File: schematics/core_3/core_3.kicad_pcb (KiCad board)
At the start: 2 copper layers, 100 x 91.1 mm, 14 parts

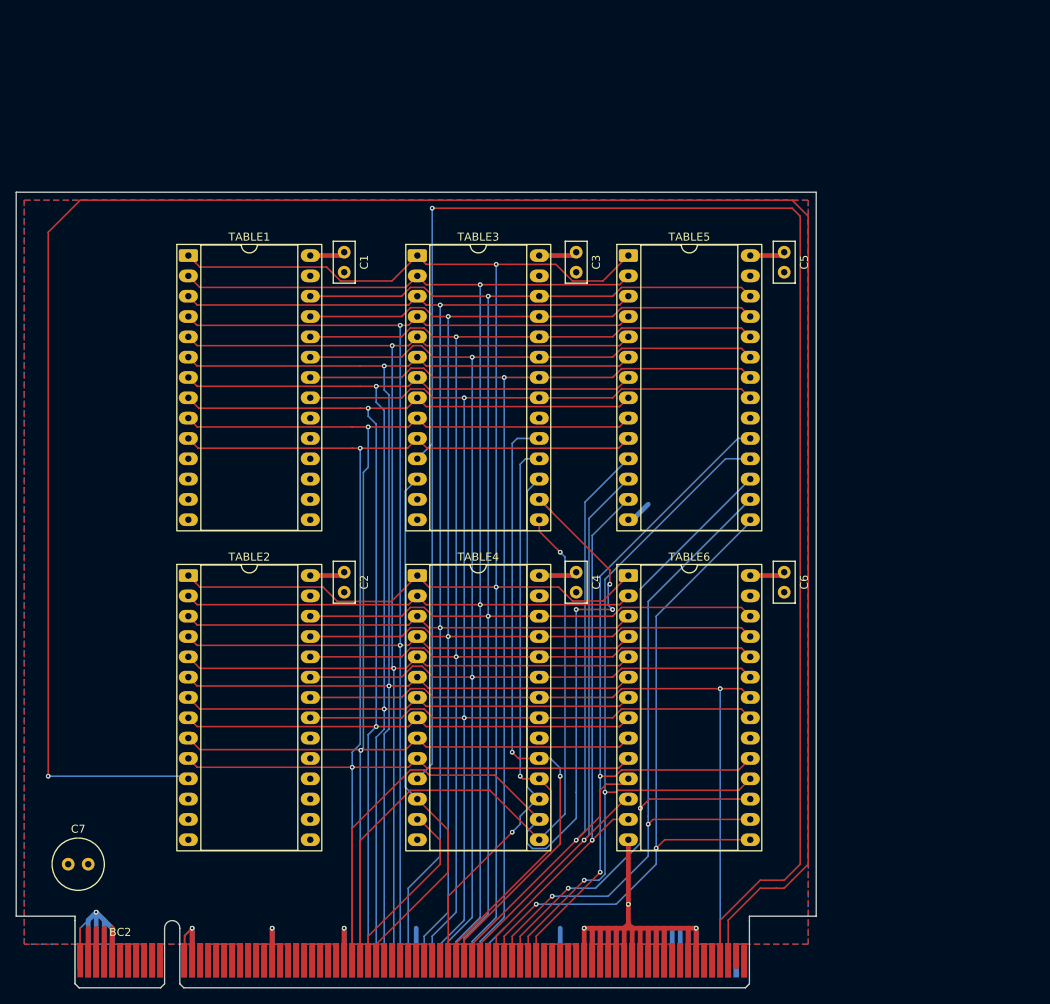
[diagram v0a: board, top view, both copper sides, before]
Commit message: tried to make core_3
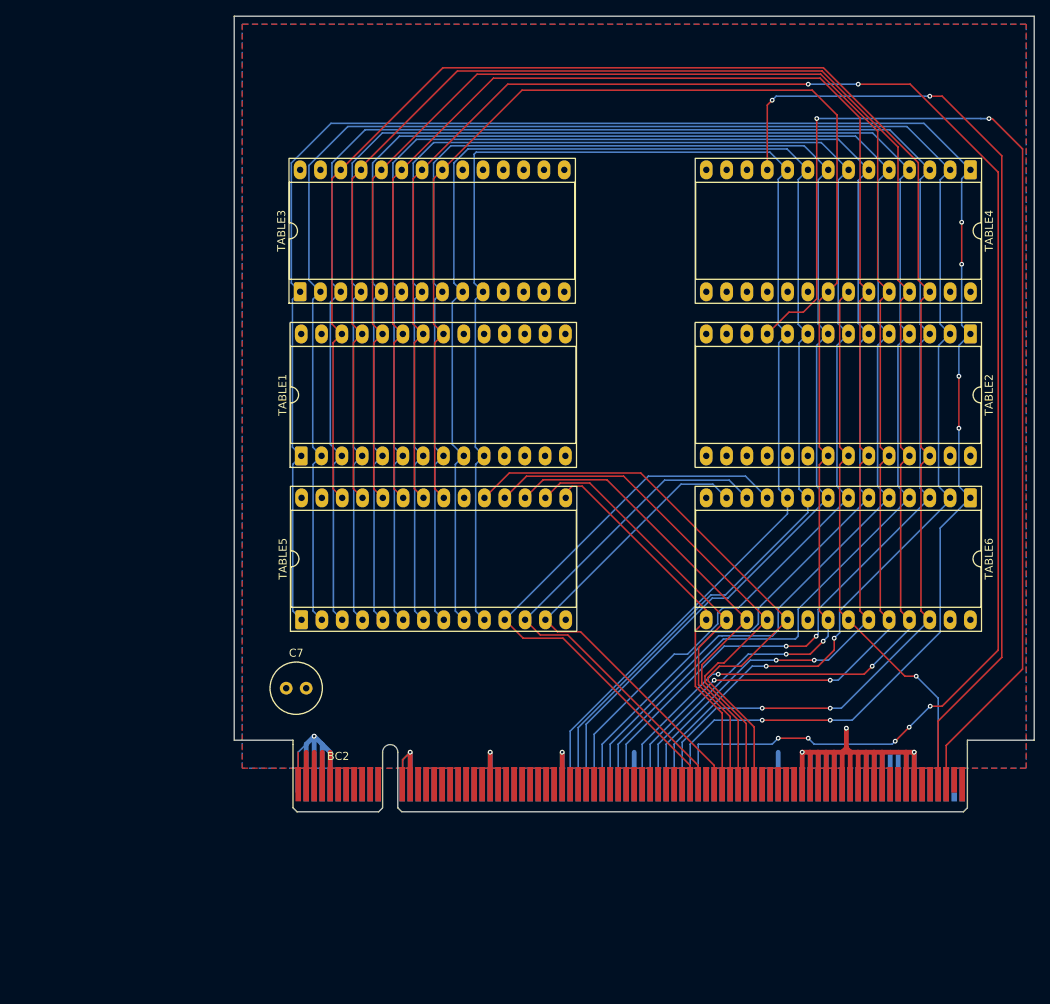
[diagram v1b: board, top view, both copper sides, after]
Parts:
- removed C1, C2, C3, C4, C5, C6: C, Capacitor_THT:C_Disc_D5.0mm_W2.5mm_P2.50mm
- moved TABLE2 102.3 mm to (172.3, 70.7), turned to -90 degrees
- moved TABLE4 85.7 mm to (172.3, 50.2), turned to -90 degrees
- moved TABLE5 61.2 mm to (88.7, 106.4), turned to 90 degrees
- moved TABLE6 43.8 mm to (172.3, 91.2), turned to -90 degrees
- moved BC2 35.0 mm to (88.2, 127.0)
- moved C7 35.0 mm to (86.8, 115.0)
- moved TABLE1 28.7 mm to (88.6, 86.0), turned to 90 degrees
- moved TABLE3 15.3 mm to (88.5, 65.4), turned to 90 degrees
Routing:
- net Net-(BC2-R4): track 282.0 -> 141.2 mm, vias 1 -> 2
- net Net-(BC2-L0): track 107.7 -> 0.00 mm, vias 3 -> 0
- net /STATE15: track 131.0 -> 233.6 mm, vias 1 -> 7
- net Net-(BC2-L4): track 220.0 -> 122.8 mm, vias 1 -> 2
- net Net-(BC2-L1): track 85.2 -> 0.00 mm, vias 1 -> 0
- net /PCIncrement: track 78.0 -> 0.00 mm, vias 2 -> 0
- net /~{Halt}: track 72.4 -> 0.00 mm, vias 1 -> 0
- net Net-(BC2-L3): track 66.7 -> 0.00 mm
- net /~{SCClear}: track 66.2 -> 0.00 mm, vias 1 -> 0
- net /STATE14: track 208.8 -> 252.2 mm, vias 2 -> 6
- net /STATE12: track 199.6 -> 241.7 mm
- net /STATE7: track 197.5 -> 238.6 mm
- net /STATE6: track 193.3 -> 231.9 mm, vias 2 -> 0
- net /ALUS3: track 86.6 -> 48.7 mm, vias 2 -> 0
- net /STATE5: track 190.9 -> 224.5 mm, vias 2 -> 0
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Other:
- board size 100 x 91.1 mm -> 100 x 91 mm
